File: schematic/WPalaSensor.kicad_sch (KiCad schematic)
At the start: 11 parts, among them J1 WeMos_mini_Hat_Left, J2 WeMos_mini_Hat_Right, J3 Fumis T01, U1 DS18B20, U2 MCP4725

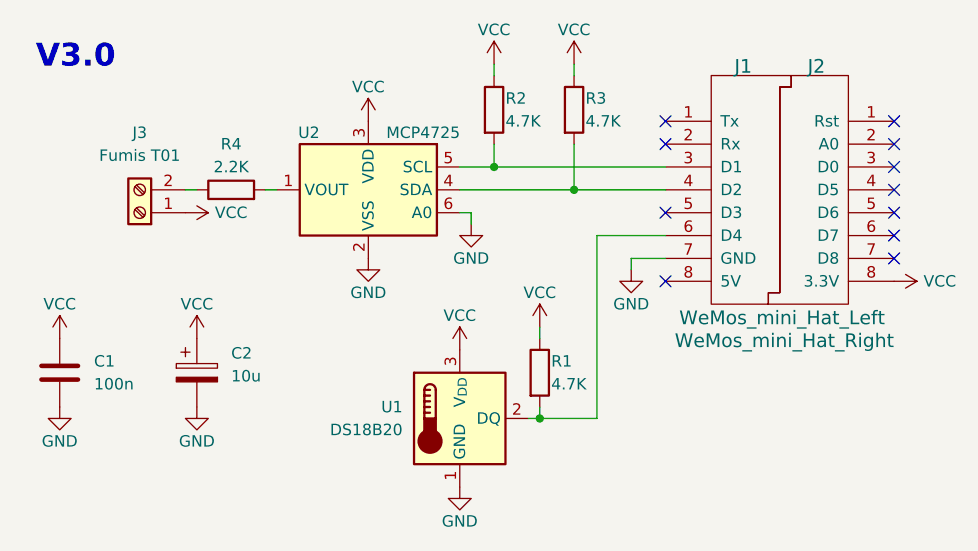
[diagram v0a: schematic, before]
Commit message: Add C3 capacitor
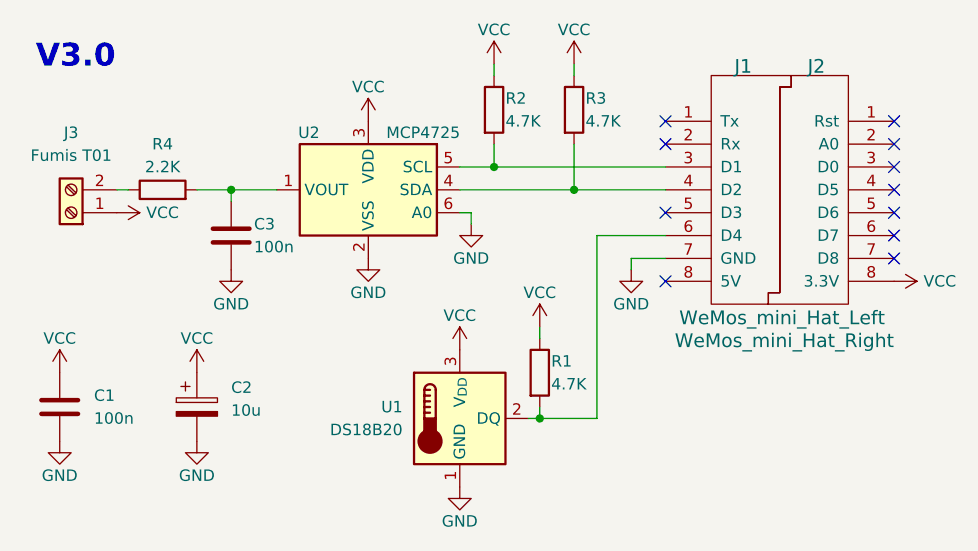
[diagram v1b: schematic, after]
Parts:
- added C3: 100n, Capacitor_SMD:C_0805_2012Metric_Pad1.18x1.45mm_HandSolder, symbol Device:C
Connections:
- net GND: now also C3.2
- net at R4.2, U2.1 (VOUT): now also C3.1
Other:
- moved on the sheet: C1, C2, J3, R4
